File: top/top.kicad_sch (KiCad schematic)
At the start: 1 part

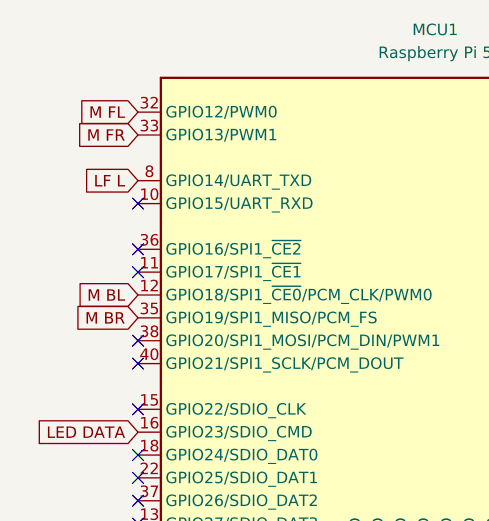
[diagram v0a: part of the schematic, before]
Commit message: lab 08/12
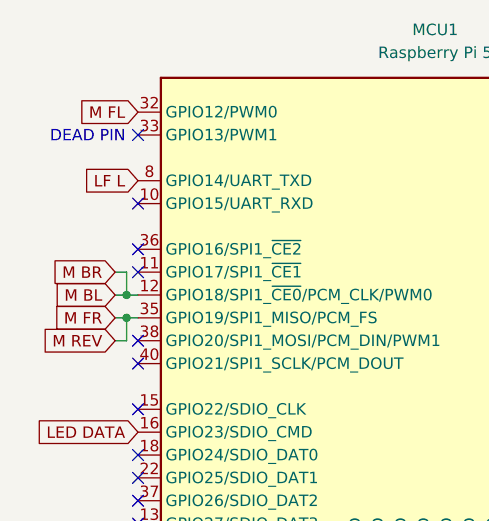
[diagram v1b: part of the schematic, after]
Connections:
- net M BR is gone; now on net M FR: MCU1.35 (GPIO19/SPI1_MISO/PCM_FS)
- net M FR: no longer MCU1.33 (GPIO13/PWM1)
- no-connect marks 24 -> 25
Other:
- note added: "DEAD PIN"
